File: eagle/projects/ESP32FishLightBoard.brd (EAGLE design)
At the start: 69.8 x 30.5 mm, 9 parts, among them U1 SN74HCT04N

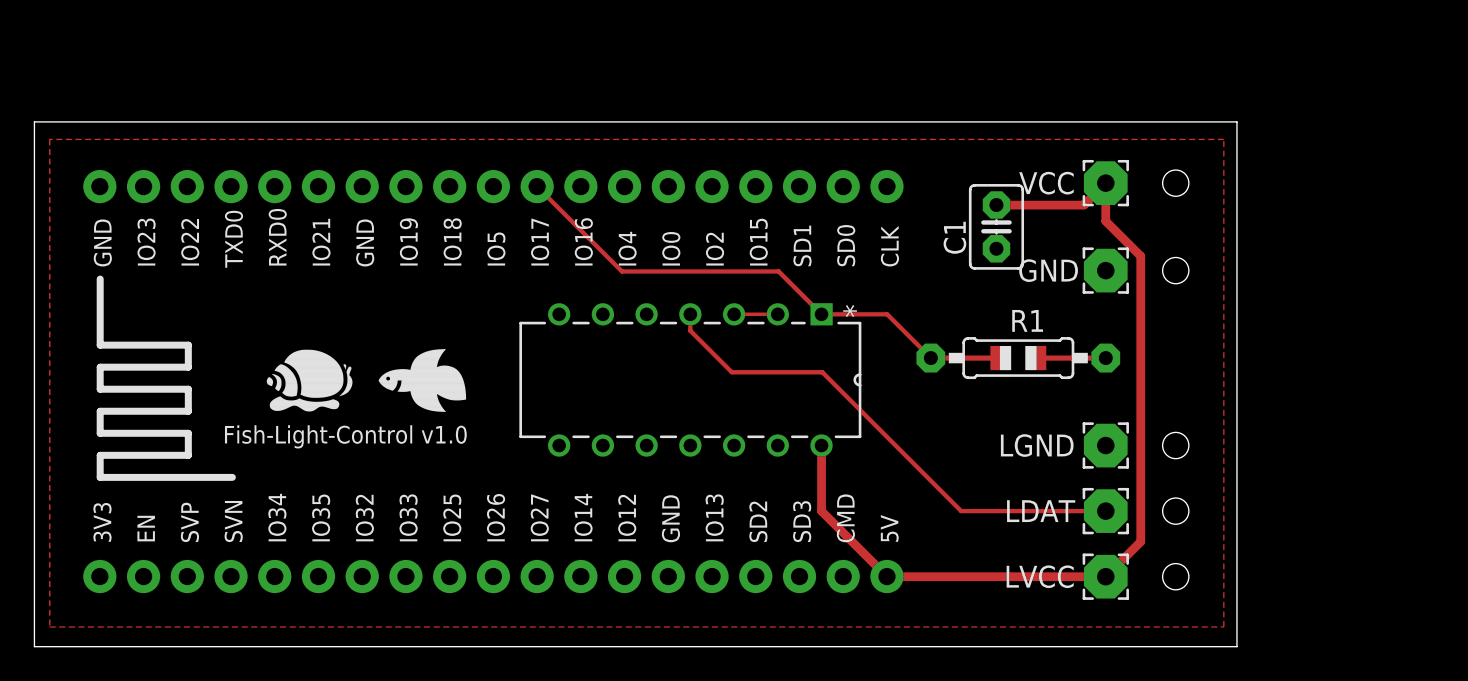
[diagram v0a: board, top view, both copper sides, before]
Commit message: updated to v1.1 PCB
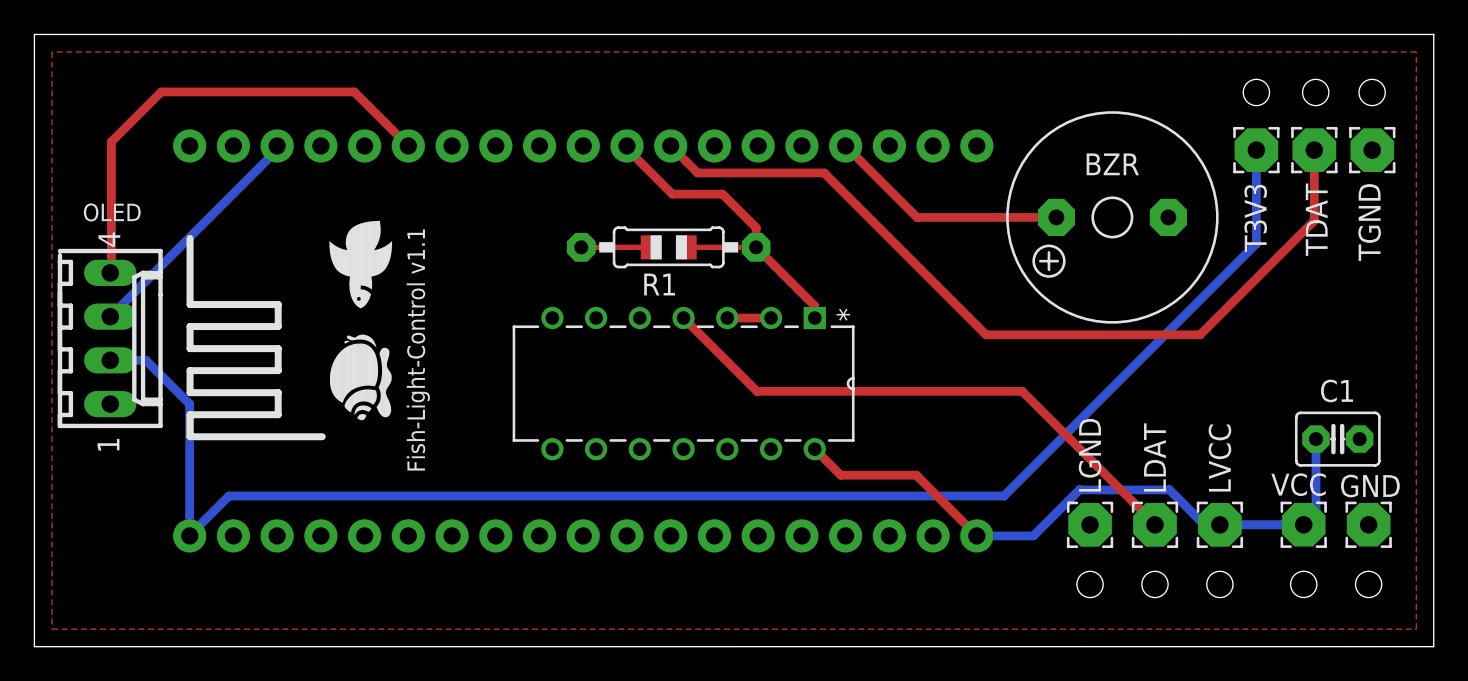
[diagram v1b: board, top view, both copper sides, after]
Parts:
- added BZR: F/QMX, buzzer:F/QMX
- added OLED: 22-27-2041-04, con-molex:6410-04
- added T3V3, TDAT, TGND: WIREPAD2,54/1,0, wirepad:2,54/1,0
- moved C1 23.3 mm to (75.7, 12.1), turned to 180 degrees
- moved VCC 22.9 mm to (73.7, 7.08), turned to 270 degrees
- moved R1 21.3 mm to (36.8, 23.2), turned to 180 degrees
- moved GND 21.2 mm to (77.5, 7.08), turned to 270 degrees
- moved LVCC 7.28 mm to (68.9, 7.08), turned to 270 degrees
- moved U$1 5.73 mm to (31.9, 17.9)
- moved LGND 4.70 mm to (61.3, 7.08), turned to 270 degrees
- moved LDAT 2.97 mm to (65.1, 7.08), turned to 270 degrees
- moved U1 0.45 mm to (30.1, 11.5)
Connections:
- new net 3V3: OLED.2, T3V3.1, U$1.1
- new net IO12: U$1.13
- new net IO14: U$1.12
- new net IO15: BZR.+, U$1.23
- new net IO16: TDAT.1, U$1.27
- new net SCL: OLED.3, U$1.36
- new net SDA: OLED.4, U$1.33
- net GND: now also BZR.-, OLED.1, TGND.1
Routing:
- net 3V3: track 0.00 -> 87.8 mm
- net IO16: track 0.00 -> 48.8 mm
- net SDA: track 0.00 -> 27.4 mm
- net VCC: track 53.3 -> 38.9 mm
- net IO15: track 0.00 -> 14.0 mm
- net SCL: track 0.00 -> 13.9 mm
- net IO17: track 27.0 -> 16.2 mm
- net IO17+: track 29.4 -> 32.4 mm
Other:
- board size 69.8 x 30.5 mm -> 81.3 x 35.6 mm
- board text added: "Fish-Light-Control v1.1"
- board text removed: "Fish-Light-Control v1.0"
